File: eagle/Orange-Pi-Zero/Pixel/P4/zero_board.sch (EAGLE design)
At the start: 13 parts, among them CN1 1X4-3.5MM, IC1 74HCT125, J1 1X2-3.5MM

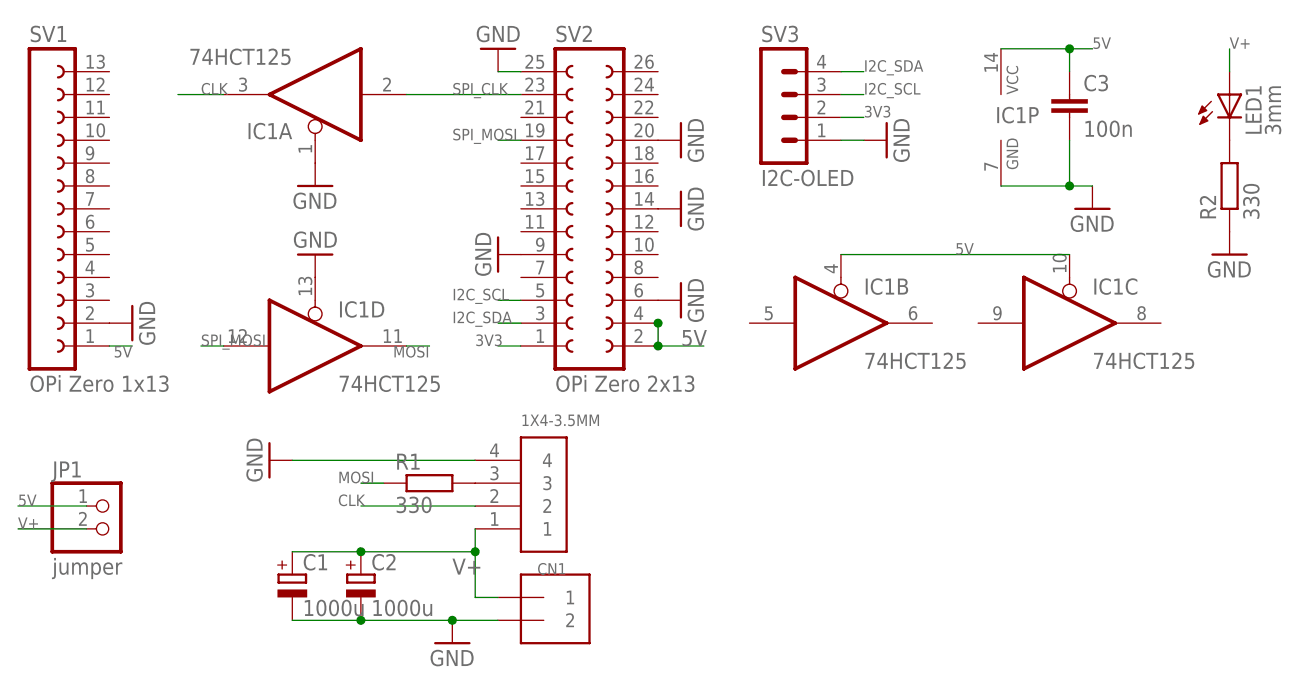
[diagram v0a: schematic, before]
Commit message: Added new gerber.zip files
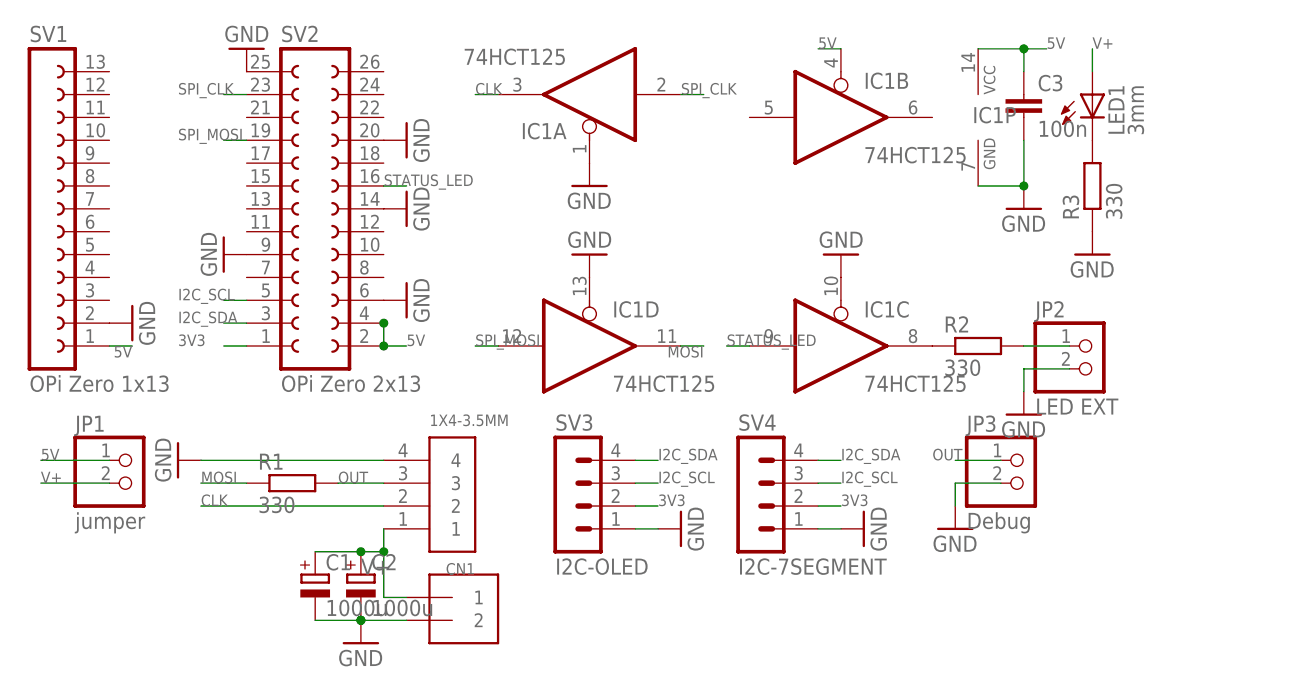
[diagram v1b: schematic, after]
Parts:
- added JP2: LED EXT, pinhead:PINHD-1X2
- added JP3: Debug, pinhead:PINHD-1X2
- added R3: 330, rcl:R-EU_0204/2V
- added SV4: I2C-7SEGMENT, con-lstb:MA04-1
- R1, R2: device rcl:R-EU_0204/7 -> rcl:R-EU_0204/2V
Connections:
- removed net N$2: CN1.3, R1.2
- new net N$3: IC1C.O, R2.1
- new net N$4: JP2.1, R2.2
- new net OUT: CN1.3, JP3.1, R1.2
- new net STATUS_LED: IC1C.I, SV2.16
- net 3V3: now also SV4.2
- net 5V: no longer IC1C.OE
- net GND: now also IC1C.OE, JP2.2, JP3.2, R3.1, SV4.1; no longer R2.1
- net I2C_SCL: now also SV4.3
- net I2C_SDA: now also SV4.4
- net N$1: now also R3.2; no longer R2.2
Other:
- moved on the sheet: C1, C3, CN1, IC1A, IC1B, IC1C, IC1D, IC1P, JP1, LED1, R1, R2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
